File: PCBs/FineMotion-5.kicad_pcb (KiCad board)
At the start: 2 copper layers, 49.9 x 19.4 mm, 43 parts, among them J1 Conn_01x02_Female, J2 Conn_01x04_Female, P1 USB_C_Plug_USB2.0, SW1 Option/FLASH Switch, SW3 SW_SPDT MAIN POWER, U1 ME6211C, U2 TP4056, U6 ESP-12F, U7 CH340C, U9 MPU-9250

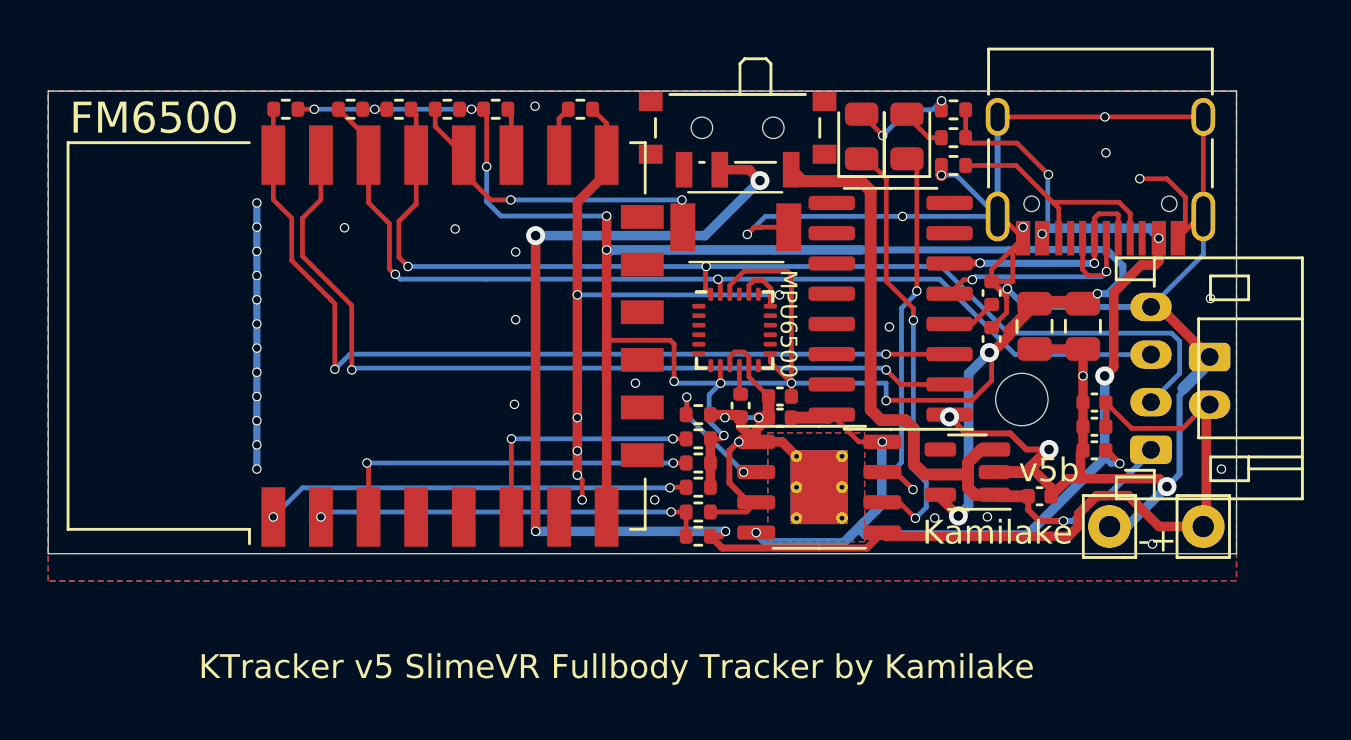
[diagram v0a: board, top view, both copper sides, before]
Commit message: Update PCB Remark
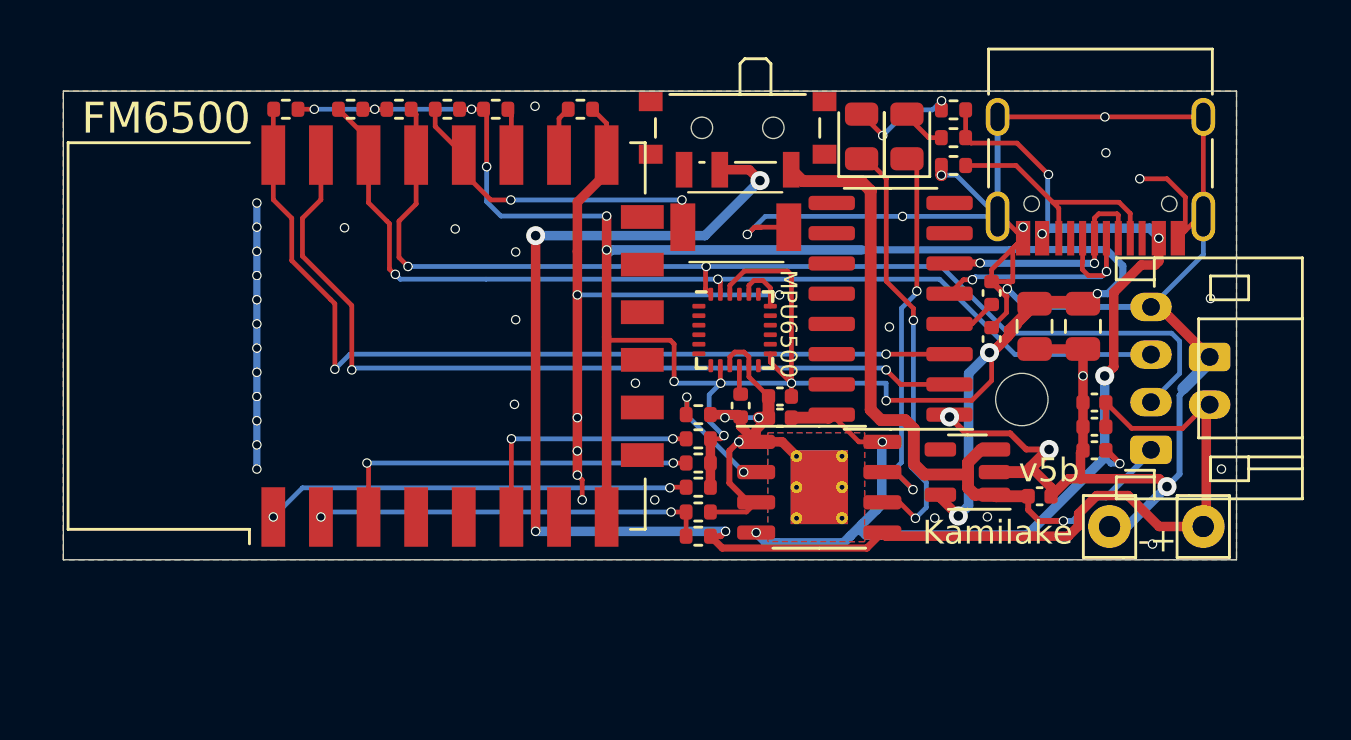
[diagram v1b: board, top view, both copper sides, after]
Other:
- board size 49.9 x 19.4 mm -> 49.3 x 19.7 mm
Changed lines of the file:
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@@
       ) (layer "B.SilkS") (width 0.01) (fill solid))
   )
-  (gr_line (start 90.17 55.753) (end 140.081 55.753) (layer "Edge.Cuts") (width 0.05))
-  (gr_line (start 140.081 55.753) (end 140.081 75.184) (layer "Edge.Cuts") (width 0.05))
-  (gr_line (start 140.081 75.184) (end 90.17 75.184) (layer "Edge.Cuts") (width 0.05))
-  (gr_line (start 90.17 75.184) (end 90.17 55.753) (layer "Edge.Cuts") (width 0.05))
+  (gr_line (start 90.805 55.753) (end 140.081 55.753) (layer "Edge.Cuts") (width 0.05))
+  (gr_line (start 140.081 55.753) (end 140.081 75.438) (layer "Edge.Cuts") (width 0.05))
+  (gr_line (start 140.081 75.438) (end 90.805 75.438) (layer "Edge.Cuts") (width 0.05))
+  (gr_line (start 90.805 75.438) (end 90.805 55.753) (layer "Edge.Cuts") (width 0.05))
   (gr_text "https://kami.live/k5" (at 99.2124 58.674) (layer "B.SilkS")
     (effects (font (size 1 1) (thickness 0.15)) (justify mirror))
@@
     (effects (font (size 1 1) (thickness 0.2)) (justify mirror))
   )
-  (gr_text "KTracker v5 SlimeVR Fullbody Tracker by Kamilake" (at 114.04 79.94) (layer "F.SilkS")
-    (effects (font (size 1 1) (thickness 0.15)))
-  )
   (gr_text "v5b" (at 132.207 71.6788) (layer "F.SilkS")
     (effects (font (size 1 1) (thickness 0.15)))
@@
     (effects (font (size 1 1) (thickness 0.15)))
   )
-  (gr_text "FM6500" (at 94.615 56.896) (layer "F.SilkS")
+  (gr_text "FM6500" (at 95.123 56.896) (layer "F.SilkS")
     (effects (font (size 1.3 1.3) (thickness 0.25)))
   )
   (gr_text "MPU6500" (at 121.2596 65.532 270) (layer "F.SilkS")
     (effects (font (size 0.7 0.7) (thickness 0.12)))
+  )
+  (gr_text "KTracker v5 SlimeVR Fullbody Tracker by Kamilake" (at 114.04 79.94) (layer "F.Fab")
+    (effects (font (size 1 1) (thickness 0.15)))
   )
   (segment (start 127.6838 58.8772) (end 127.6838 59.2816) (width 0.5) (layer "F.Cu") (net 1))
@@
     (polygon
       (pts
-        (xy 140.08 76.32)
-        (xy 90.17 76.33)
-        (xy 90.17 55.75)
+        (xy 140.07982 75.431)
+        (xy 90.80482 75.441)
+        (xy 90.805 55.75)
         (xy 140.08 55.75)
       )
@@
       (pts
         (xy 98.515 76.327)
-        (xy 90.17 76.327)
-        (xy 90.17 55.753)
+        (xy 90.805 76.327)
+        (xy 90.805 55.753)
         (xy 98.515 55.753)
       )
